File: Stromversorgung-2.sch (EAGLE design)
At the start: 16 parts, among them U1 TSR2-2450, U2 TSR1-2433, U3 TSR1-2425, X1 Ein/Aus, X2 MAC64L, X3 Ein/Aus

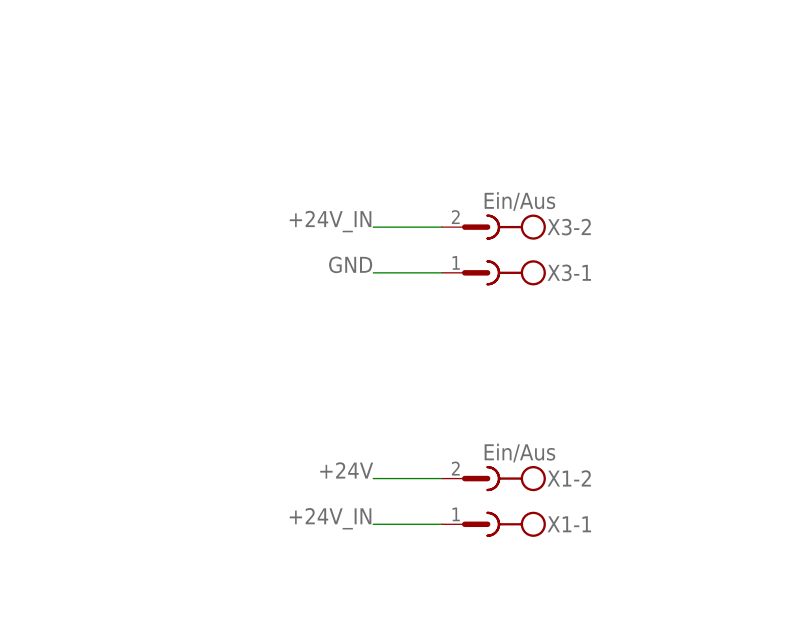
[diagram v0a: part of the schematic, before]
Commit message: Layouts angepasst
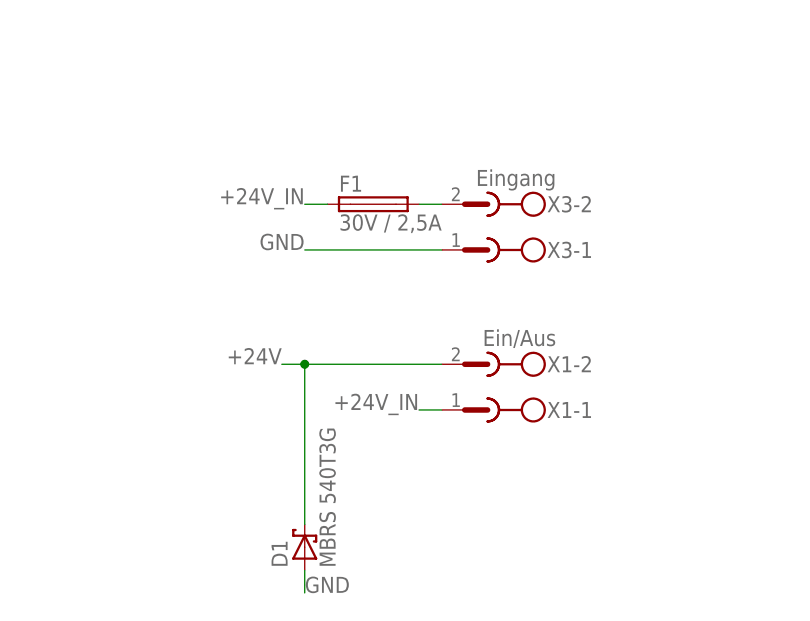
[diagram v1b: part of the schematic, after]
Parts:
- added D1: MBRS 540T3G, diode:SCHOTTKY-DIODESMC
- added F1: 30V / 2,5A, fuse:LITTLEFUSE
- X3: value Ein/Aus -> Eingang
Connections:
- new net +24V_IN_RAW: F1.2, X3-2.1
- net +24V: now also D1.C
- net +24V_IN: now also F1.1; no longer X3-2.1
- net GND: now also D1.A
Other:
- moved on the sheet: X1-1, X1-2, X3-1, X3-2
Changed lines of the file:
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@@
 <part name="R4" library="rcl" deviceset="R-EU_" device="R1206" value="12k"/>
 <part name="LED4" library="led" deviceset="LED" device="3MM" value="2mA ge"/>
-<part name="X3" library="con-phoenix-508" deviceset="MSTBA2" device="" value="Ein/Aus"/>
+<part name="X3" library="con-phoenix-508" deviceset="MSTBA2" device="" value="Eingang"/>
+<part name="D1" library="diode" deviceset="SCHOTTKY-DIODE" device="SMC" value="MBRS 540T3G"/>
+<part name="F1" library="fuse" deviceset="LITTLEFUSE" device="" value="30V / 2,5A"/>
 </parts>
 <sheets>
@@
 </plain>
 <instances>
-<instance part="X1" gate="-1" x="132.08" y="12.7" rot="R180"/>
-<instance part="X1" gate="-2" x="132.08" y="17.78" rot="R180"/>
+<instance part="X1" gate="-1" x="132.08" y="25.4" rot="R180"/>
+<instance part="X1" gate="-2" x="132.08" y="30.48" rot="R180"/>
 <instance part="LED1" gate="G$1" x="185.42" y="40.64"/>
 <instance part="LED2" gate="G$1" x="205.74" y="40.64"/>
@@
 <instance part="R4" gate="G$1" x="243.84" y="50.8" rot="R90"/>
 <instance part="LED4" gate="G$1" x="243.84" y="40.64"/>
-<instance part="X3" gate="-1" x="132.08" y="40.64" rot="R180"/>
-<instance part="X3" gate="-2" x="132.08" y="45.72" rot="R180"/>
+<instance part="X3" gate="-1" x="132.08" y="43.18" rot="R180"/>
+<instance part="X3" gate="-2" x="132.08" y="48.26" rot="R180"/>
+<instance part="D1" gate="G$1" x="111.76" y="10.16" rot="R90"/>
+<instance part="F1" gate="A" x="119.38" y="48.26"/>
 </instances>
 <busses>
@@
 <segment>
 <pinref part="X1" gate="-2" pin="1"/>
-<wire x1="127" y1="17.78" x2="119.38" y2="17.78" width="0.1524" layer="91"/>
-<label x="119.38" y="17.78" size="1.778" layer="95" rot="MR0"/>
+<wire x1="127" y1="30.48" x2="111.76" y2="30.48" width="0.1524" layer="91"/>
+<label x="109.22" y="30.48" size="1.778" layer="95" rot="MR0"/>
+<pinref part="D1" gate="G$1" pin="C"/>
+<wire x1="111.76" y1="30.48" x2="109.22" y2="30.48" width="0.1524" layer="91"/>
+<wire x1="111.76" y1="12.7" x2="111.76" y2="30.48" width="0.1524" layer="91"/>
+<junction x="111.76" y="30.48"/>
 </segment>
 </net>
@@
 </segment>
 <segment>
+<label x="111.76" y="43.18" size="1.778" layer="95" rot="MR0"/>
 <pinref part="X3" gate="-1" pin="1"/>
-<wire x1="127" y1="40.64" x2="119.38" y2="40.64" width="0.1524" layer="91"/>
-<label x="119.38" y="40.64" size="1.778" layer="95" rot="MR0"/>
+<wire x1="111.76" y1="43.18" x2="127" y2="43.18" width="0.1524" layer="91"/>
+</segment>
+<segment>
+<pinref part="D1" gate="G$1" pin="A"/>
+<wire x1="111.76" y1="7.62" x2="111.76" y2="5.08" width="0.1524" layer="91"/>
+<label x="111.76" y="5.08" size="1.778" layer="95"/>
 </segment>
 </net>
@@
 <net name="+24V_IN" class="0">
 <segment>
+<pinref part="X1" gate="-1" pin="1"/>
+<label x="124.46" y="25.4" size="1.778" layer="95" rot="MR0"/>
+<wire x1="124.46" y1="25.4" x2="127" y2="25.4" width="0.1524" layer="91"/>
+</segment>
+<segment>
+<pinref part="F1" gate="A" pin="1"/>
+<wire x1="111.76" y1="48.26" x2="114.3" y2="48.26" width="0.1524" layer="91"/>
+<label x="111.76" y="48.26" size="1.778" layer="95" rot="MR0"/>
+</segment>
+</net>
+<net name="+24V_IN_RAW" class="0">
+<segment>
 <pinref part="X3" gate="-2" pin="1"/>
-<wire x1="127" y1="45.72" x2="119.38" y2="45.72" width="0.1524" layer="91"/>
-<label x="119.38" y="45.72" size="1.778" layer="95" rot="MR0"/>
-</segment>
-<segment>
-<pinref part="X1" gate="-1" pin="1"/>
-<wire x1="119.38" y1="12.7" x2="127" y2="12.7" width="0.1524" layer="91"/>
-<label x="119.38" y="12.7" size="1.778" layer="95" rot="MR0"/>
-</segment>
-</net>
+<pinref part="F1" gate="A" pin="2"/>
+<wire x1="124.46" y1="48.26" x2="127" y2="48.26" width="0.1524" layer="91"/>
+</segment>
+</net>
